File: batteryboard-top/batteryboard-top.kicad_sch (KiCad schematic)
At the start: 6 parts, among them J1 Conn_02x05_Odd_Even, J2 Conn_02x05_Odd_Even

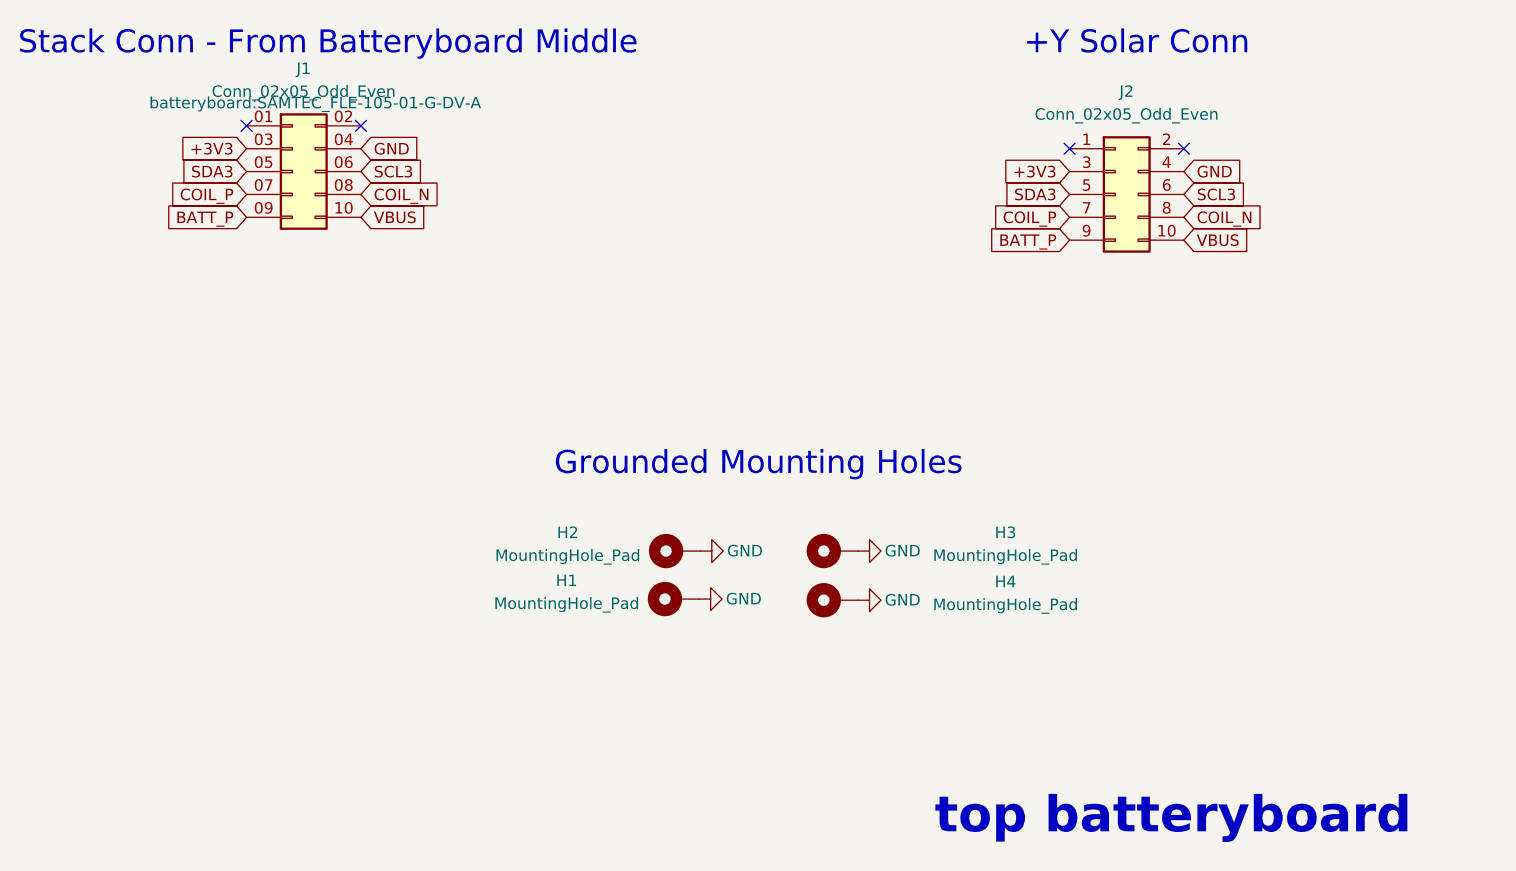
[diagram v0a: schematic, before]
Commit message: Fixes and cleanup
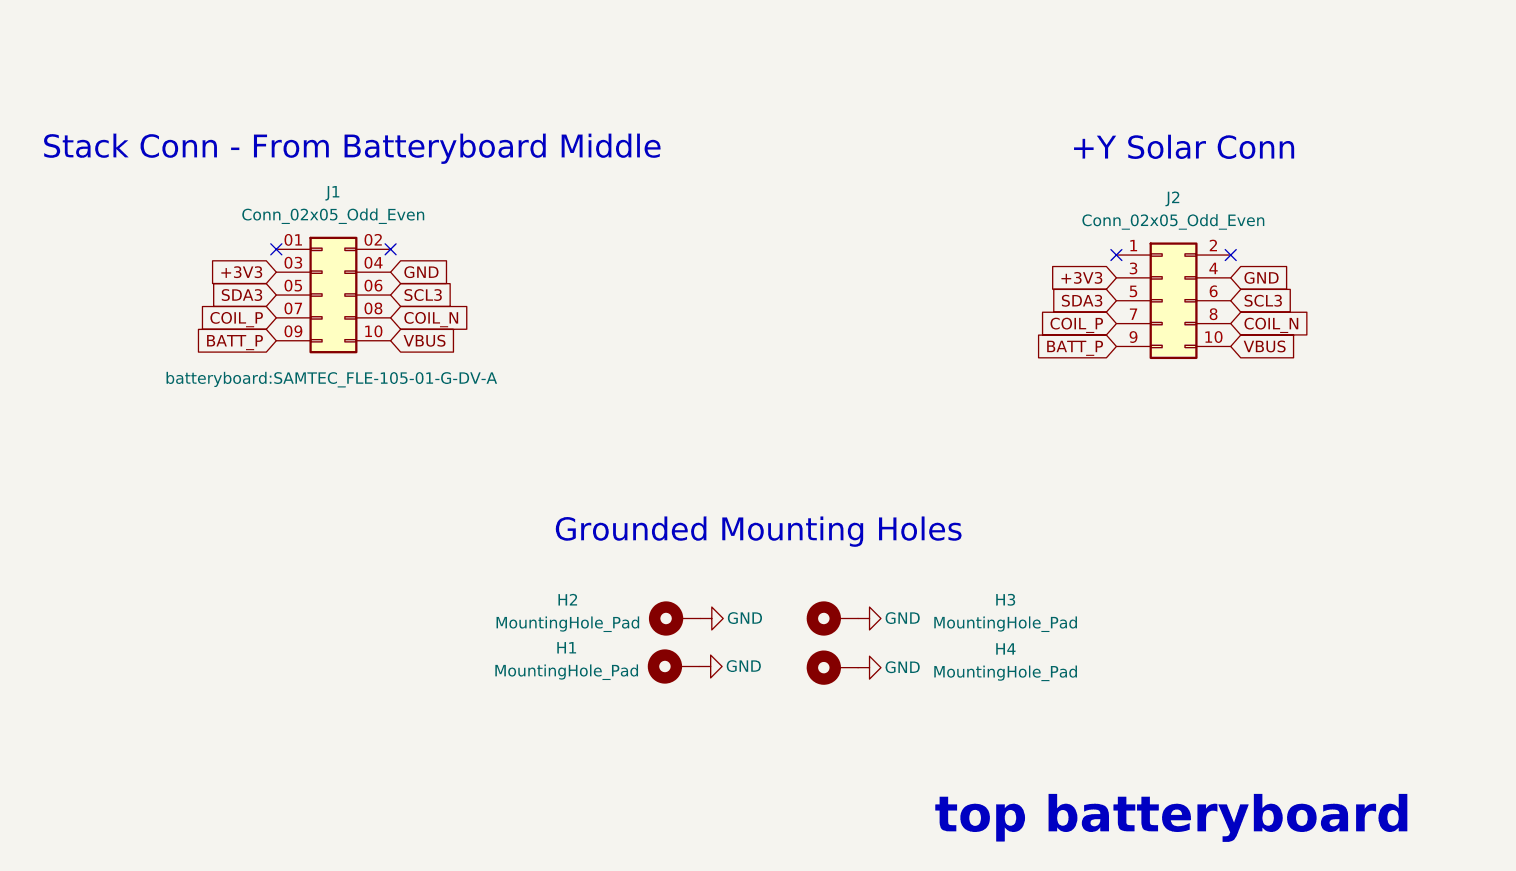
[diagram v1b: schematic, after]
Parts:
- J2: footprint batteryboard:SAMTEC-FTS-105-01-X-DV -> batteryboard:FTS-105-XX-YY-DV-A
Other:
- moved on the sheet: H1, H2, H3, H4, J1, J2
